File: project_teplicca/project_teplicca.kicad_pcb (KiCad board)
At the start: 2 copper layers, 99.9 x 52.7 mm, 33 parts, among them J3 Relay_conn, J6 Relay_conn_term, U1 AMS1117-3.3

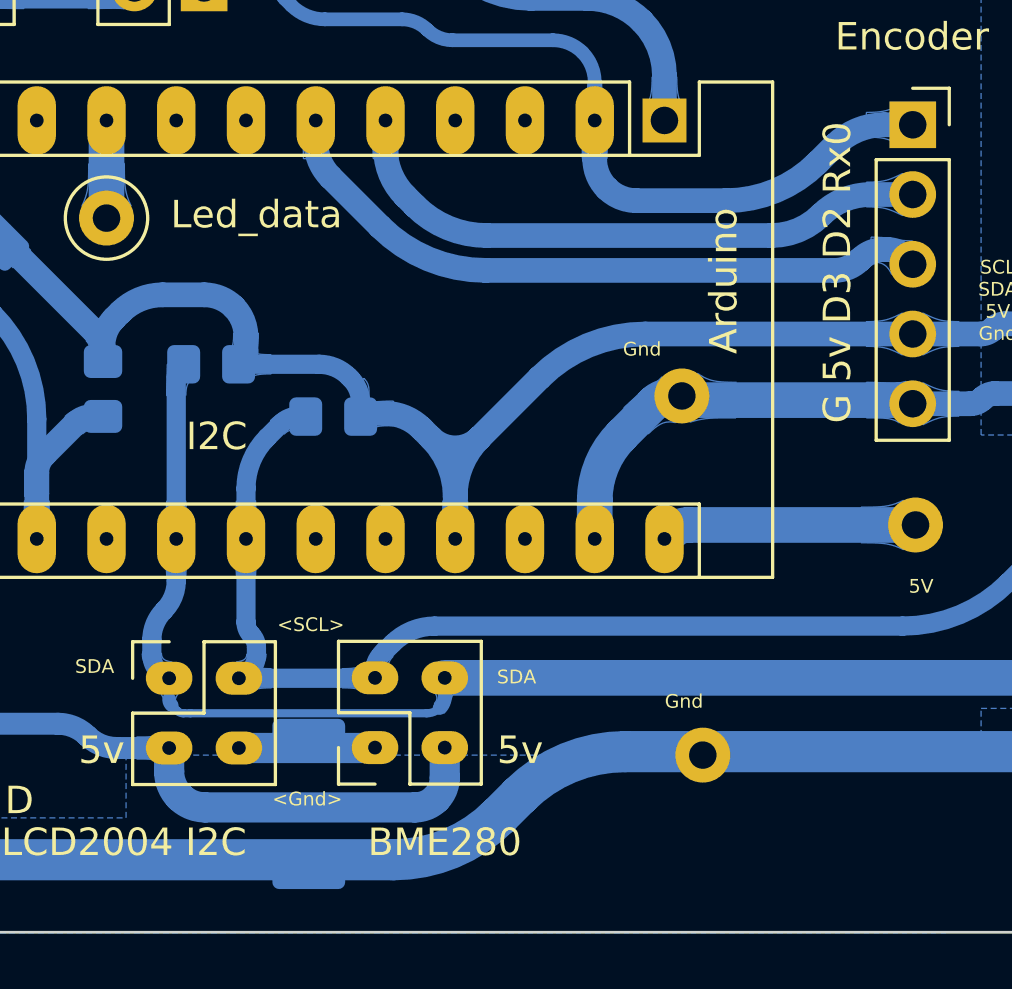
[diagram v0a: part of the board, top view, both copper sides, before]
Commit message: d
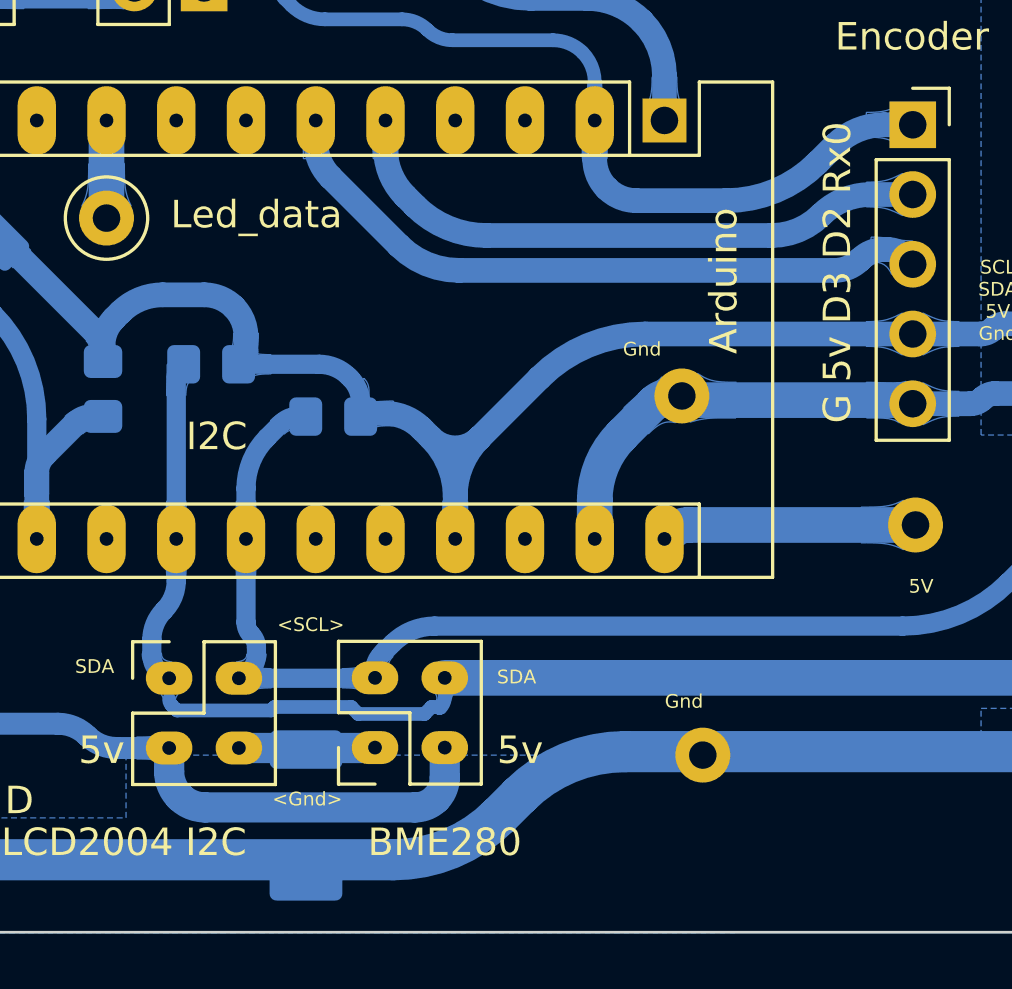
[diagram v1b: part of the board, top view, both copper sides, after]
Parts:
- moved REF** 0.43 mm to (151.4, 131.3)
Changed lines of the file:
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@@
   )
   (footprint "Resistor_SMD:R_2010_5025Metric_Pad1.40x2.65mm_HandSolder" (layer "B.Cu")
-    (at 151.4856 130.9116 -90)
+    (at 151.384 131.331 -90)
     (descr "Resistor SMD 2010 (5025 Metric), square (rectangular) end terminal, IPC_7351 nominal with elongated pad for handsoldering. (Body size source: IPC-SM-782 page 72, https://www.pcb-3d.com/wordpress/wp-content/uploads/ipc-sm-782a_amendment_1_and_2.pdf), generated with kicad-footprint-generator")
     (tags "resistor handsolder")
@@
   (arc (start 154.2796 107.0356) (mid 154.466311 107.974261) (end 154.99802 108.77002) (width 0.9) (layer "B.Cu") (net 5))
   (arc (start 171.943017 108.7166) (mid 170.967014 108.910738) (end 170.1396 109.4636) (width 0.9) (layer "B.Cu") (net 5))
-  (segment (start 170.631784 111.4806) (end 157.930563 111.4806) (width 0.9) (layer "B.Cu") (net 6))
+  (segment (start 170.631784 111.4806) (end 156.959211 111.4806) (width 0.9) (layer "B.Cu") (net 6))
   (segment (start 151.7396 106.7816) (end 151.7396 106.0196) (width 0.9) (layer "B.Cu") (net 6))
-  (segment (start 152.278415 108.082415) (end 154.082807 109.886807) (width 0.9) (layer "B.Cu") (net 6))
+  (segment (start 152.278415 108.082415) (end 154.769657 110.573657) (width 0.9) (layer "B.Cu") (net 6))
   (segment (start 173.2126 110.9876) (end 173.4816 111.2566) (width 0.9) (layer "B.Cu") (net 6))
   (segment (start 171.551599 111.099599) (end 171.575157 111.076042) (width 0.9) (layer "B.Cu") (net 6))
@@
   (arc (start 173.2126 110.9876) (mid 172.914641 110.78851) (end 172.563176 110.7186) (width 0.9) (layer "B.Cu") (net 6))
   (arc (start 171.551599 111.099599) (mid 171.129584 111.381581) (end 170.631784 111.4806) (width 0.9) (layer "B.Cu") (net 6))
-  (arc (start 154.082807 109.886807) (mid 155.848172 111.066386) (end 157.930563 111.4806) (width 0.9) (layer "B.Cu") (net 6))
+  (arc (start 154.769657 110.573657) (mid 155.774233 111.244893) (end 156.959211 111.4806) (width 0.9) (layer "B.Cu") (net 6))
   (arc (start 172.4381 110.7186) (mid 171.971078 110.811496) (end 171.575157 111.076042) (width 0.9) (layer "B.Cu") (net 6))
   (arc (start 151.7396 106.7816) (mid 151.879633 107.485596) (end 152.278415 108.082415) (width 0.9) (layer "B.Cu") (net 6))
@@
   (arc (start 127.4191 96.1771) (mid 127.06742 95.942115) (end 126.652587 95.8596) (width 0.7) (layer "B.Cu") (net 19))
   (arc (start 138.617392 111.677392) (mid 136.852026 110.497813) (end 134.769636 110.0836) (width 0.7) (layer "B.Cu") (net 19))
+  (segment (start 146.685 127.508) (end 150.114 127.508) (width 0.5) (layer "B.Cu") (net 21))
   (segment (start 180.970807 110.8851) (end 179.0841 110.8851) (width 1.3) (layer "B.Cu") (net 21))
+  (segment (start 153.035 127.381) (end 153.289 127.635) (width 0.5) (layer "B.Cu") (net 21))
   (segment (start 145.7706 124.936217) (end 145.7706 125.475925) (width 0.7) (layer "B.Cu") (net 21))
   (segment (start 146.4006 126.8426) (end 146.4006 126.3981) (width 0.3) (layer "B.Cu") (net 21))
-  (segment (start 147.1676 127.6096) (end 146.9136 127.6096) (width 0.3) (layer "B.Cu") (net 21))
+  (segment (start 150.114 127.508) (end 150.241 127.381) (width 0.5) (layer "B.Cu") (net 21))
+  (segment (start 155.956 127.381) (end 156.21 127.381) (width 0.5) (layer "B.Cu") (net 21))
+  (segment (start 153.289 127.635) (end 155.702 127.635) (width 0.5) (layer "B.Cu") (net 21))
   (segment (start 177.902283 126.3196) (end 156.4386 126.3196) (width 1.3) (layer "B.Cu") (net 21))
+  (segment (start 156.21 127.381) (end 156.2481 127.4191) (width 0.5) (layer "B.Cu") (net 21))
   (segment (start 146.4006 126.8426) (end 146.4006 127.0966) (width 0.3) (layer "B.Cu") (net 21))
+  (segment (start 150.241 127.381) (end 153.035 127.381) (width 0.5) (layer "B.Cu") (net 21))
+  (segment (start 155.702 127.635) (end 155.956 127.381) (width 0.5) (layer "B.Cu") (net 21))
   (segment (start 146.6596 121.2596) (end 146.6596 115.360518) (width 0.7) (layer "B.Cu") (net 21))
-  (segment (start 156.4386 126.959192) (end 156.4386 126.3196) (width 0.5) (layer "B.Cu") (net 21))
-  (segment (start 147.1676 127.6096) (end 155.788192 127.6096) (width 0.3) (layer "B.Cu") (net 21))
   (segment (start 182.8546 112.768892) (end 182.8546 121.367283) (width 1.3) (layer "B.Cu") (net 21))
   (segment (start 146.0221 126.0831) (end 146.228698 126.289698) (width 0.7) (layer "B.Cu") (net 21))
   (segment (start 146.6596 121.2596) (end 146.6596 122.789982) (width 0.7) (layer "B.Cu") (net 21))
-  (segment (start 146.490402 127.313402) (end 146.696797 127.519797) (width 0.3) (layer "B.Cu") (net 21))
+  (segment (start 146.490402 127.313402) (end 146.685 127.508) (width 0.5) (layer "B.Cu") (net 21))
+  (segment (start 156.4386 126.959192) (end 156.4386 126.3196) (width 0.5) (layer "B.Cu") (net 21))
   (segment (start 146.7946 115.0346) (end 146.9296 114.8996) (width 0.7) (layer "B.Cu") (net 21))
   (arc (start 146.4006 126.3981) (mid 146.382001 126.353198) (end 146.3371 126.3346) (width 0.3) (layer "B.Cu") (net 21))
+  (arc (start 156.2481 127.4191) (mid 156.38909 127.208092) (end 156.4386 126.959192) (width 0.5) (layer "B.Cu") (net 21))
   (arc (start 182.8546 121.367283) (mid 182.477627 123.262452) (end 181.4041 124.8691) (width 1.3) (layer "B.Cu") (net 21))
   (arc (start 182.30285 111.43685) (mid 182.711204 112.047996) (end 182.8546 112.768892) (width 1.3) (layer "B.Cu") (net 21))
   (arc (start 182.30285 111.43685) (mid 181.691703 111.028495) (end 180.970807 110.8851) (width 1.3) (layer "B.Cu") (net 21))
   (arc (start 146.7946 115.0346) (mid 146.694685 115.184132) (end 146.6596 115.360518) (width 0.7) (layer "B.Cu") (net 21))
-  (arc (start 156.2481 127.4191) (mid 156.037092 127.56009) (end 155.788192 127.6096) (width 0.3) (layer "B.Cu") (net 21))
   (arc (start 146.2151 123.8631) (mid 145.886121 124.35545) (end 145.7706 124.936217) (width 0.7) (layer "B.Cu") (net 21))
+  (arc (start 145.7706 125.475925) (mid 145.835962 125.804525) (end 146.0221 126.0831) (width 0.7) (layer "B.Cu") (net 21))
   (arc (start 146.4006 127.0966) (mid 146.423938 127.213932) (end 146.490402 127.313402) (width 0.5) (layer "B.Cu") (net 21))
-  (arc (start 145.7706 125.475925) (mid 145.835962 125.804525) (end 146.0221 126.0831) (width 0.7) (layer "B.Cu") (net 21))
-  (arc (start 146.696797 127.519797) (mid 146.796267 127.58626) (end 146.9136 127.6096) (width 0.3) (layer "B.Cu") (net 21))
-  (arc (start 156.4386 126.959192) (mid 156.38909 127.208092) (end 156.2481 127.4191) (width 0.5) (layer "B.Cu") (net 21))
   (arc (start 146.6596 122.789982) (mid 146.544078 123.370749) (end 146.2151 123.8631) (width 0.7) (layer "B.Cu") (net 21))
   (arc (start 181.4041 124.8691) (mid 179.797452 125.942627) (end 177.902283 126.3196) (width 1.3) (layer "B.Cu") (net 21))
